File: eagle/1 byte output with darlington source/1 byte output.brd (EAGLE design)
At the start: 160 x 100 mm, 8 parts, among them IC1 74LS595N, IC2 74LS595N, X1 MKDSN1,5/9-5,08, X2 MKDSN1,5/8-5,08, X3 MKDSN1,5/5-5,08, X4 MKDSN1,5/5-5,08

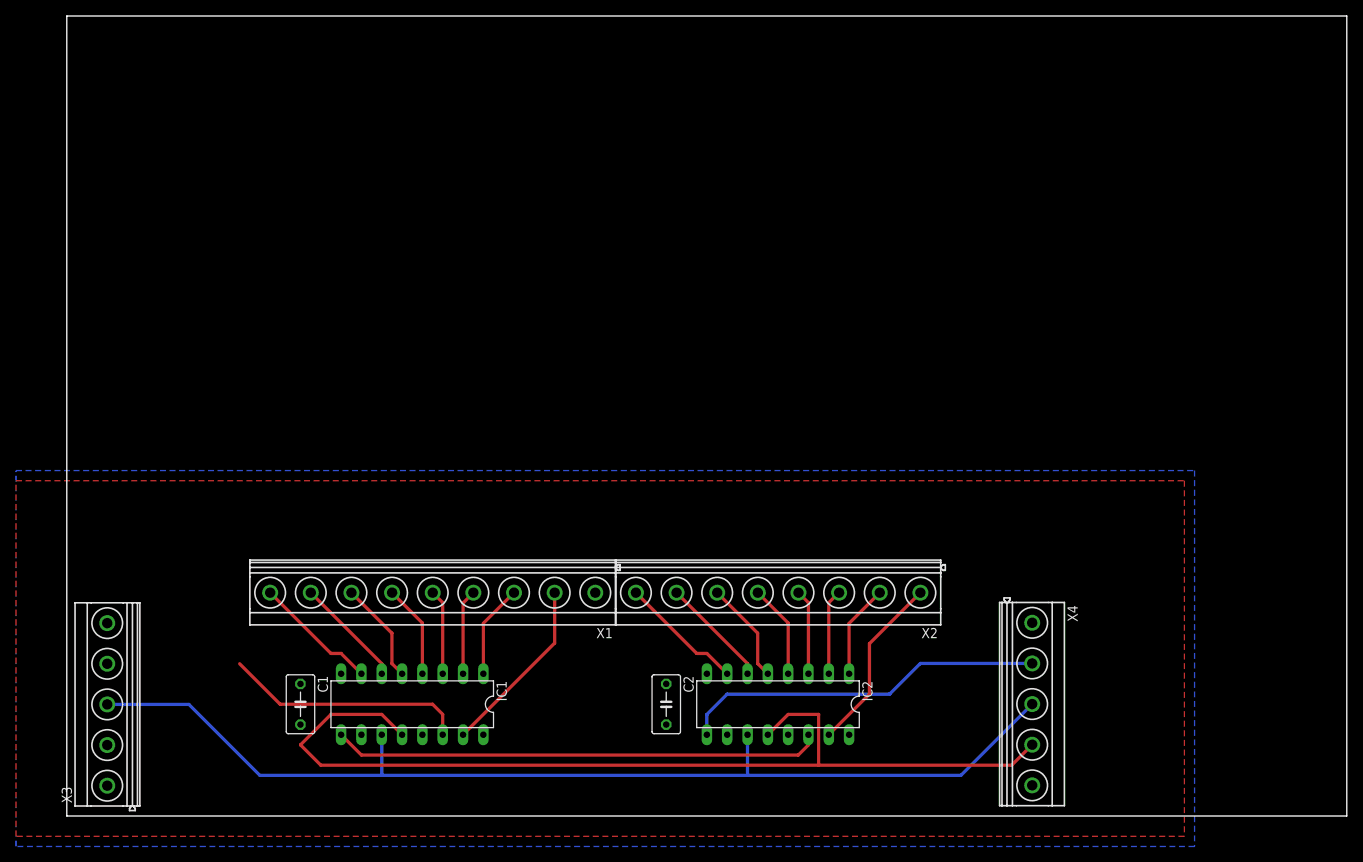
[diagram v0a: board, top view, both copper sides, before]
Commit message: periodic check-in
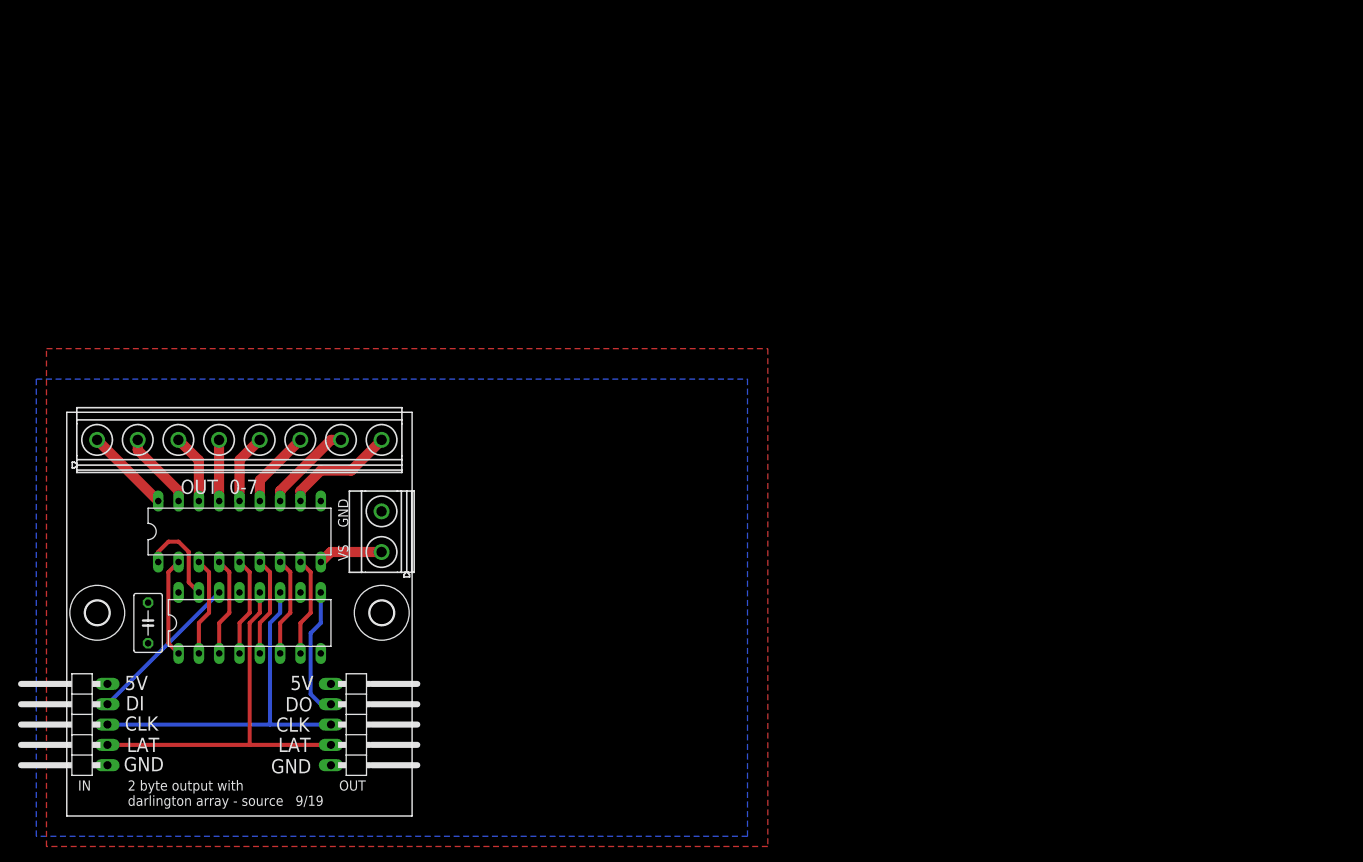
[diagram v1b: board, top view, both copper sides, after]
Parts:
- removed C2: (no value), resistor:C050-035X075
- removed IC2: 74LS595N, 74xx-us:DIL16
- removed X2: MKDSN1,5/8-5,08, con-phoenix-508:MKDSN1,5/8-5,08
- removed X3, X4: MKDSN1,5/5-5,08, con-phoenix-508:MKDSN1,5/5-5,08
- added H1, H2: MOUNT-HOLE3.0, holes:3,0
- added IC3: MIC2981A, uln-udn:DIL18
- added JP1, JP2: (no value), pinhead:1X05/90
- added X5: MKDSN1,5/2-5,08, con-phoenix-508:MKDSN1,5/2-5,08
- X1: value MKDSN1,5/9-5,08 -> MKDSN1,5/8-5,08; device con-phoenix-508:MKDSN1,5/9-5,08 -> con-phoenix-508:MKDSN1,5/8-5,08
- moved X1 30.7 mm to (21.6, 47.0), turned to 0 degrees
- moved IC1 22.7 mm to (22.9, 24.1), turned to 0 degrees
- moved C1 21.6 mm to (10.2, 24.1)
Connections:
- removed net DP: IC1.9, IC2.14
- removed net QA0: IC1.15, X1.2
- removed net QA1: IC1.1, X1.3
- removed net QA2: IC1.2, X1.4
- removed net QA3: IC1.3, X1.5
- removed net QA4: IC1.4, X1.6
- removed net QA5: IC1.5, X1.7
- removed net QA6: IC1.6, X1.8
- removed net QA7: IC1.7, X1.9
- removed net QB0: IC2.15, X2.1
- removed net QB1: IC2.1, X2.2
- removed net QB2: IC2.2, X2.3
- removed net QB3: IC2.3, X2.4
- removed net QB4: IC2.4, X2.5
- removed net QB5: IC2.5, X2.6
- removed net QB6: IC2.6, X2.7
- removed net QB7: IC2.7, X2.8
- new net N$1: IC3.15, X1.4
- new net N$17: IC1.15, IC3.1
- new net N$18: IC1.1, IC3.2
- new net N$19: IC1.2, IC3.3
- new net N$2: IC3.16, X1.3
- new net N$20: IC1.3, IC3.4
- new net N$21: IC1.4, IC3.5
- new net N$22: IC1.5, IC3.6
- new net N$23: IC1.6, IC3.7
- new net N$24: IC1.7, IC3.8
- new net N$3: IC3.17, X1.2
- new net N$4: IC3.18, X1.1
- new net N$5: IC3.14, X1.5
- new net N$6: IC3.12, X1.7
- new net N$7: IC3.11, X1.8
- new net N$8: IC3.13, X1.6
- new net VS: IC3.9, X5.1
- net CLK: now also JP1.3, JP2.3; no longer IC2.11, X3.3, X4.3
- net DI: now also JP1.4; no longer X3.4
- net DO: now also IC1.9, JP2.2; no longer IC2.9, X4.2
- net GND: now also IC3.10, JP1.1, JP2.5, X5.2; no longer C2.2, IC2.13, IC2.8, X1.1, X3.1, X4.5
- net LATCH: now also JP1.2, JP2.4; no longer IC2.12, X3.2, X4.4
- net VCC: now also JP1.5, JP2.1; no longer C2.1, IC2.10, IC2.16, X3.5, X4.1
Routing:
- net CLK: track 133.1 -> 45.0 mm
- net LATCH: track 122.6 -> 47.5 mm
- net DP: track 61.3 -> 0.00 mm
- net DO: track 45.8 -> 16.3 mm
- net QB0: track 22.5 -> 0.00 mm
- net QA0: track 22.5 -> 0.00 mm
- net QB7: track 15.6 -> 0.00 mm
- net QA7: track 15.6 -> 0.00 mm
- net N$7: track 0.00 -> 14.1 mm
- net QB6: track 13.8 -> 0.00 mm
- net QA6: track 13.8 -> 0.00 mm
- net QA5: track 12.8 -> 0.00 mm
- net QB5: track 12.8 -> 0.00 mm
- net N$18: track 0.00 -> 12.5 mm
- net N$24: track 0.00 -> 12.5 mm
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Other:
- board size 160 x 100 mm -> 43.2 x 50.5 mm
- board text added: "2 byte output with darlington array - source 9/19"
- board text added: "5V"
- board text added: "CLK"
- board text added: "DI"
- board text added: "DO"
- board text added: "GND"
- board text added: "IN"
- board text added: "LAT"
- board text added: "OUT"
- board text added: "OUT 0-7"
- board text added: "VS"
